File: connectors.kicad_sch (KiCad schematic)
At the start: 10 parts, among them J3 09665526612, J5 5747841-4

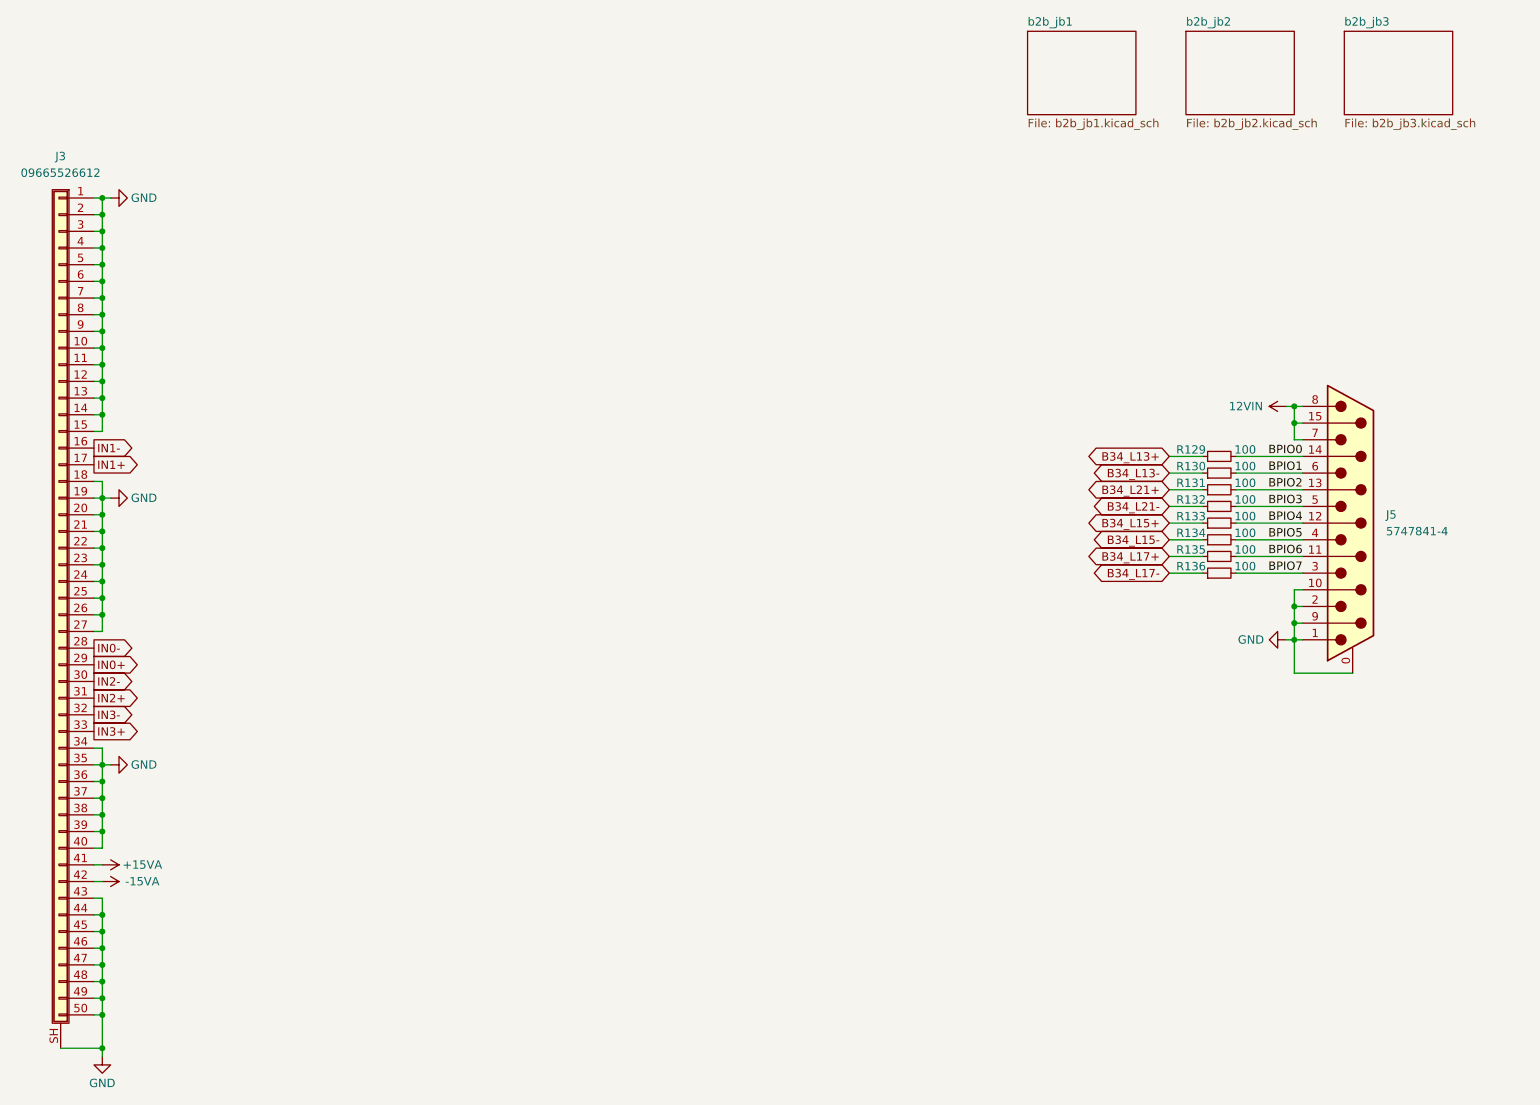
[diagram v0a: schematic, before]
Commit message: edit README.md
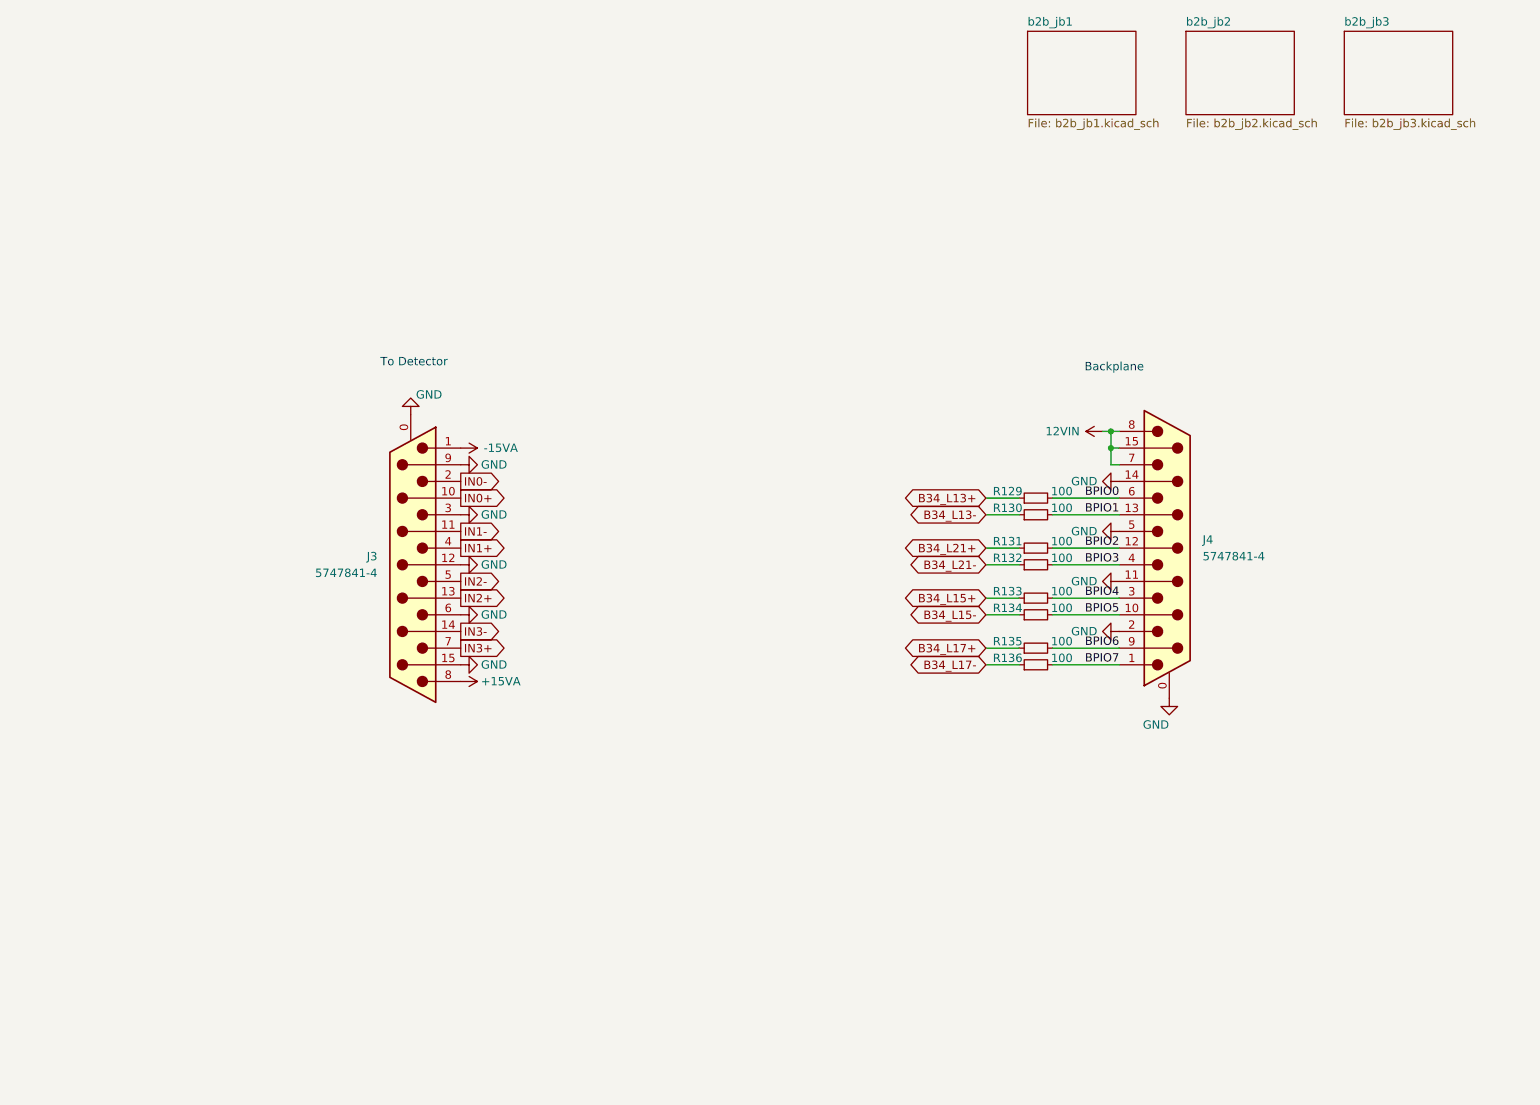
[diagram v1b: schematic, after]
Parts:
- removed J3: 09665526612, lib:09665526612, symbol Connector_Generic_Shielded:Conn_01x50_Shielded
- added J3: 5747841-4, lib:57478414, symbol Connector:DA15_Pins_MountingHoles
- renumbered J5 to J4
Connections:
- net +15VA: now also J3.8
- net -15VA: now also J3.1
- net BPIO0: now also J4.6; no longer J4.14 (P14)
- net BPIO1: now also J4.13 (P13); no longer J4.6
- net BPIO2: now also J4.12 (P12); no longer J4.13 (P13)
- net BPIO3: now also J4.4; no longer J4.5
- net BPIO4: now also J4.3; no longer J4.12 (P12)
- net BPIO5: now also J4.10 (P10); no longer J4.4
- net BPIO6: now also J4.9 (P9); no longer J4.11 (P111)
- net BPIO7: now also J4.1; no longer J4.3
- net GND: now also J4.11 (P111), J4.14 (P14), J4.5, J3.0 (PAD), J3.12 (P12), J3.15 (P15), J3.3, J3.6, J3.9 (P9); no longer J4.1, J4.10 (P10), J4.9 (P9)
- net IN0+: now also J3.10 (P10)
- net IN0-: now also J3.2
- net IN1+: now also J3.4
- net IN1-: now also J3.11 (P111)
- net IN2+: now also J3.13 (P13)
- net IN2-: now also J3.5
- net IN3+: now also J3.7
- net IN3-: now also J3.14 (P14)
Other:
- note added: "Backplane"
- note added: "To Detector"
- company: (none) -> NOIRLab
- title: (none) -> 4 channel ADC Module
- moved on the sheet: J4, R129, R130, R131, R132, R133, R134, R135, R136
